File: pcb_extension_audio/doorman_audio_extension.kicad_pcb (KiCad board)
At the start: 4 copper layers, 31.4 x 29.6 mm, 39 parts, among them J1 Audio Out CH2, J4 Conn_02x07_Odd_Even, J5 Audio In CH2, U1 ES8388

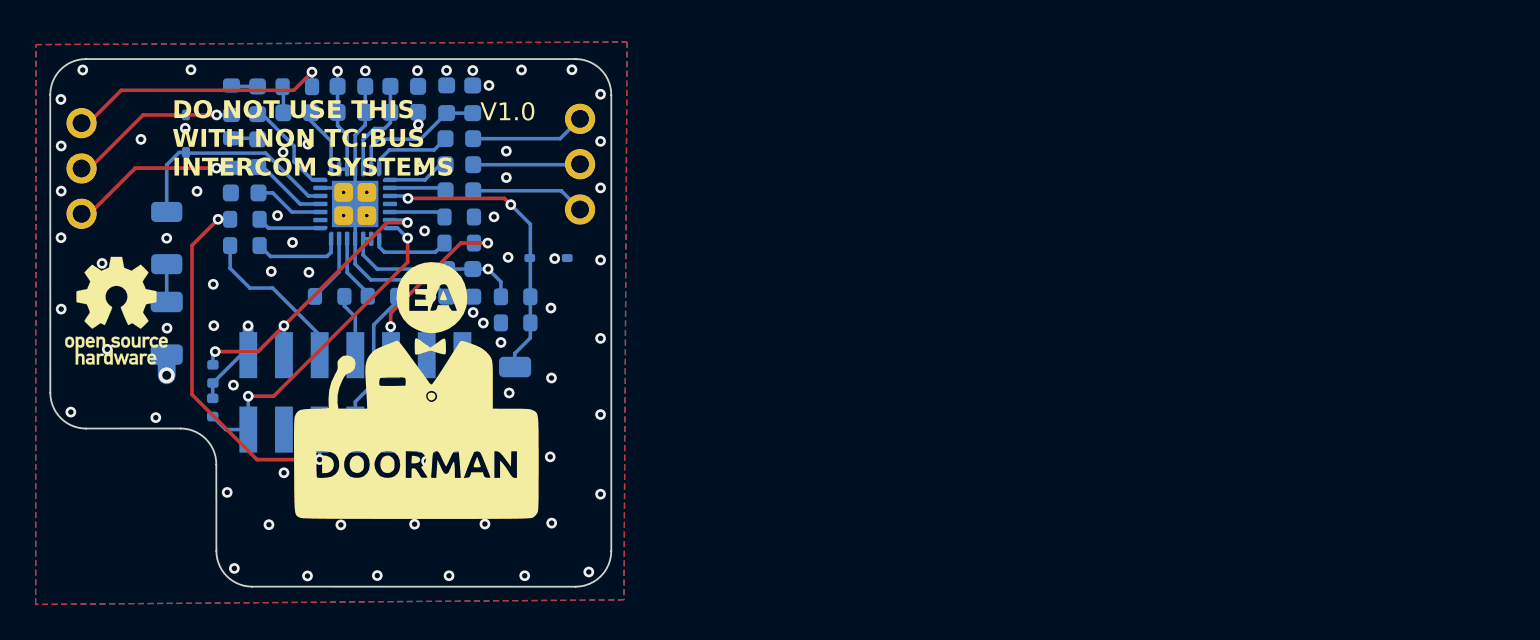
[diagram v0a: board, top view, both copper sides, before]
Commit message: WIP
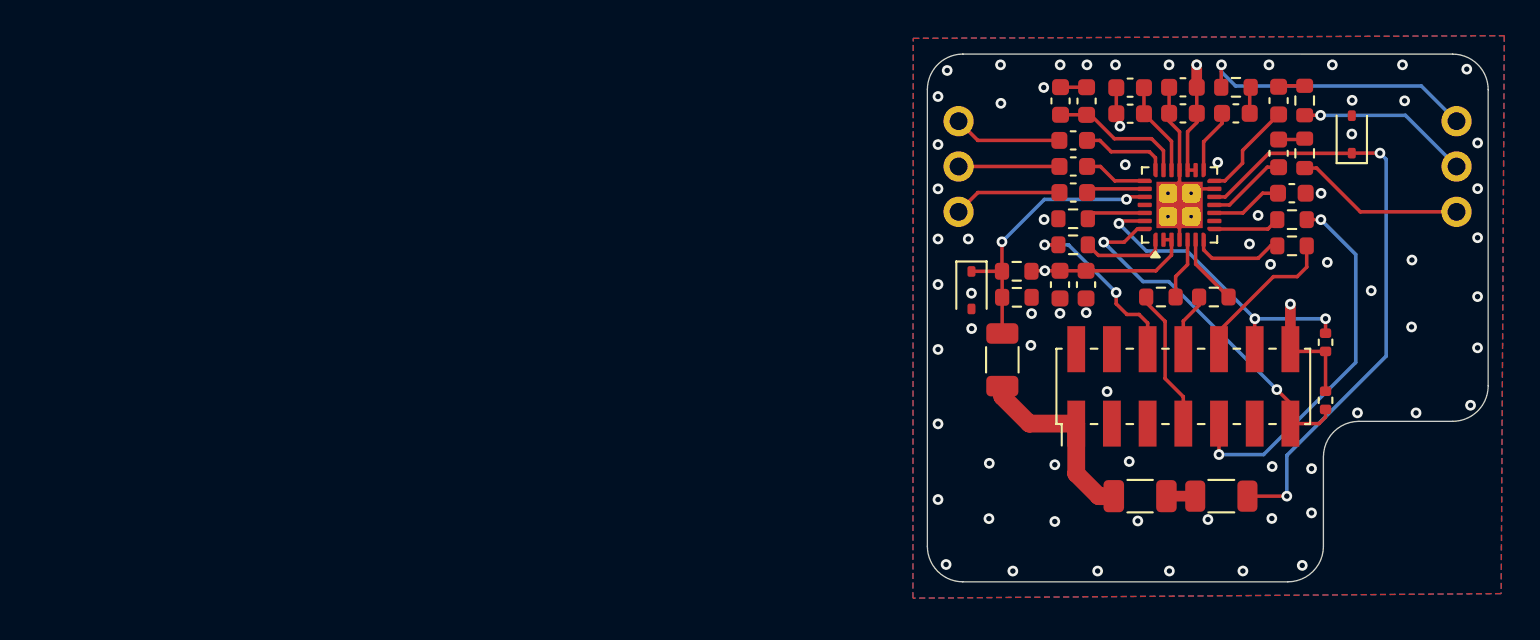
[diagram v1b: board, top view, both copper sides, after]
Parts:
- C1, C10: value 0.1uF -> 100nF; moved to F.Cu
- C11, C12, C13, C14, C17, C18, C19, C2, C20, C21, C3, C4, C5, C6, C7, D1, D2, R1, R13, R14, R15, R16, R17, R18, R19, R2, R20, R21, R3, R5, R6, U1: moved to F.Cu
- G***, REF**: moved to B.Cu
- J1: value Audio Out CH2 -> Audio Out; moved to B.Cu
- J4: value Conn_02x07_Odd_Even -> Extension Board Connector; moved to F.Cu
- J5: value Audio In CH2 -> Audio In; moved to B.Cu
- moved J1 77.0 mm to (205.6, 86.3), turned to 180 degrees
- moved REF** 72.6 mm to (203.1, 98.6), turned to 180 degrees
- moved D2 65.3 mm to (199.8, 87.0)
- moved R13 62.4 mm to (198.3, 98.7)
- moved R14 62.4 mm to (198.3, 101.9)
- moved R6 60.8 mm to (192.4, 107.3), turned to 180 degrees
- moved R1 60.1 mm to (197.1, 88.1)
- moved R3 60.1 mm to (197.1, 85.1)
- moved R17 58.7 mm to (196.4, 93.3), turned to 0 degrees
- moved R19 58.7 mm to (196.4, 91.8), turned to 0 degrees
- moved C17 58.7 mm to (196.4, 90.3), turned to 180 degrees
- moved C13 57.2 mm to (195.7, 85.1)
- moved C6 57.2 mm to (195.7, 88.1)
- moved C14 55.3 mm to (187.9, 107.3), turned to 0 degrees
- moved C7 52.6 mm to (193.3, 85.8), turned to 0 degrees
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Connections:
- J5 pad 1: AUDIO_IN_R1 -> AUDIO_IN_R2
- J5 pad 3: AUDIO_IN_R2 -> AUDIO_IN_R1
- U1 pad : GND -> (no net)
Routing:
- net AUDIO_OUT_L1: track 12.5 -> 34.2 mm, vias 0 -> 2
- net BUS_WIRE2: track 26.1 -> 10.8 mm, vias 2 -> 0
- net GND: track 18.9 -> 12.3 mm, vias 70 -> 68
- net +3.3V: track 56.0 -> 53.0 mm
- net I2C_CLK: track 18.8 -> 20.5 mm
- net AUDIO_IN_L1: track 17.0 -> 16.0 mm
- net AUDIO_OUT_L2: track 15.1 -> 16.0 mm
- net I2C_DAT: track 17.2 -> 17.8 mm
- net Net-(C14-Pad2): track 2.12 -> 1.61 mm
- net AUDIO_OUT_R1: track 9.69 -> 9.53 mm, vias 1 -> 0
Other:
- outline, holes or cut-outs redrawn
- board text added: "PCB3D_BR_doorman_ea"
- board text added: "PCB3D_TL_doorman_ea"
- board text removed: "PCB3D_BR_doorman"
- board text removed: "PCB3D_TL_doorman"
